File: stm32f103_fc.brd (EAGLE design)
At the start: 55.5 x 74.9 mm, 47 parts, among them IC1 STM32F10XCXT6, IC2 LD1117AS33TR, U2 9DoF IMU, Y1 8MHz, Y2 32.768MHz

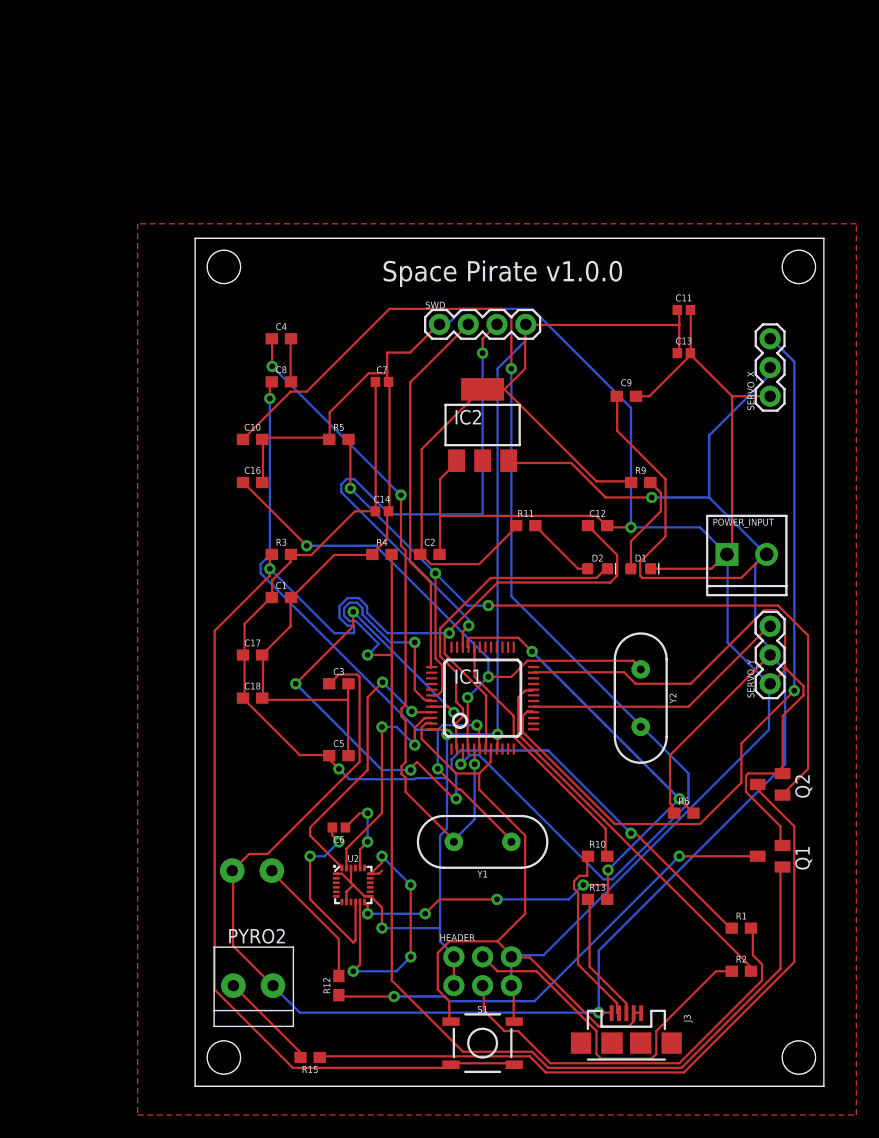
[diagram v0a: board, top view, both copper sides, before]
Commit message: done version 2
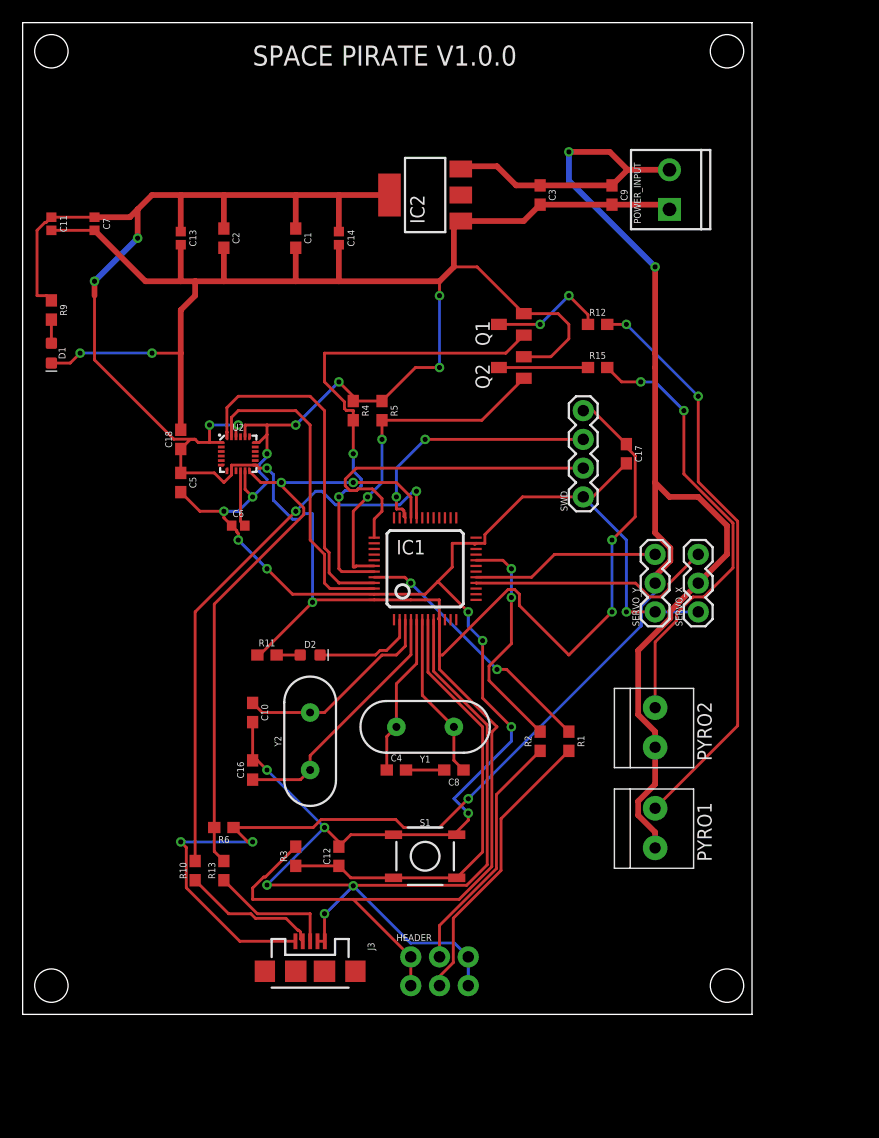
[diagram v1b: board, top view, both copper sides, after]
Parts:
- moved R15 66.0 mm to (58.4, 68.6), turned to 0 degrees
- moved R12 62.7 mm to (58.4, 72.4), turned to 0 degrees
- moved C11 56.4 mm to (10.2, 81.3), turned to 270 degrees
- moved D1 55.4 mm to (10.2, 69.8), turned to 270 degrees
- moved R9 54.3 mm to (10.2, 73.7), turned to 270 degrees
- moved Q1 52.3 mm to (50.8, 72.4)
- moved C3 46.7 mm to (53.3, 83.8), turned to 270 degrees
- moved C13 45.6 mm to (21.6, 80.0), turned to 270 degrees
- moved Q2 43.3 mm to (50.8, 68.6)
- moved PYRO2 42.3 mm to (63.5, 36.8), turned to 270 degrees
- moved R6 40.7 mm to (25.4, 27.9), turned to 180 degrees
- moved C4 39.4 mm to (40.6, 33.0)
- moved U2 39.4 mm to (26.7, 61.0)
- moved C8 37.5 mm to (45.7, 33.0), turned to 180 degrees
- moved C17 37.5 mm to (61.0, 61.0), turned to 270 degrees
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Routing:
- net RESET: track 129.6 -> 40.4 mm, vias 2 -> 0
- net PC14: track 107.4 -> 18.6 mm, vias 2 -> 0
- net PB7: track 110.6 -> 43.6 mm
- net N$13: track 63.7 -> 7.87 mm
- net BOOT0: track 77.5 -> 22.8 mm, vias 6 -> 2
- net PB6: track 77.0 -> 30.0 mm, vias 3 -> 2
- net PA6: track 68.8 -> 22.0 mm, vias 1 -> 0
- net N$7: track 60.7 -> 14.4 mm, vias 3 -> 0
- net N$9: track 57.3 -> 14.8 mm, vias 3 -> 0
- net N$14: track 11.8 -> 51.5 mm, vias 0 -> 2
- net VCC3V3: track 207.3 -> 240.2 mm, vias 4 -> 8
- net N$15: track 42.6 -> 10.5 mm
- net N$12: track 8.81 -> 39.8 mm, vias 0 -> 2
- net PC15: track 51.3 -> 22.4 mm, vias 3 -> 0
- net SWDIO: track 50.6 -> 22.6 mm
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- removed copper zone on layer 1, net GND
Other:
- board size 55.5 x 74.9 mm -> 64.4 x 87.6 mm
- board text added: "SPACE PIRATE V1.0.0"
- board text removed: "Space Pirate v1.0.0"
